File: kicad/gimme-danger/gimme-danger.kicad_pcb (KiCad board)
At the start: 4 copper layers, 46.1 x 30 mm, 74 parts, among them J3 Screw_Terminal_01x06, Q1 AO3400A, Q2 AO3400A, Q3 AO3400A, Q4 AO3400A, U1 ESP32-S3-WROOM-1, U2 TPD6S300RUKR, U3 U261-241N-4BS2SS, U4 AO4407A, U5 SKRKAEE020, U6 DDTC143EUA, U7 SKRKAEE020, U8 TPS54302

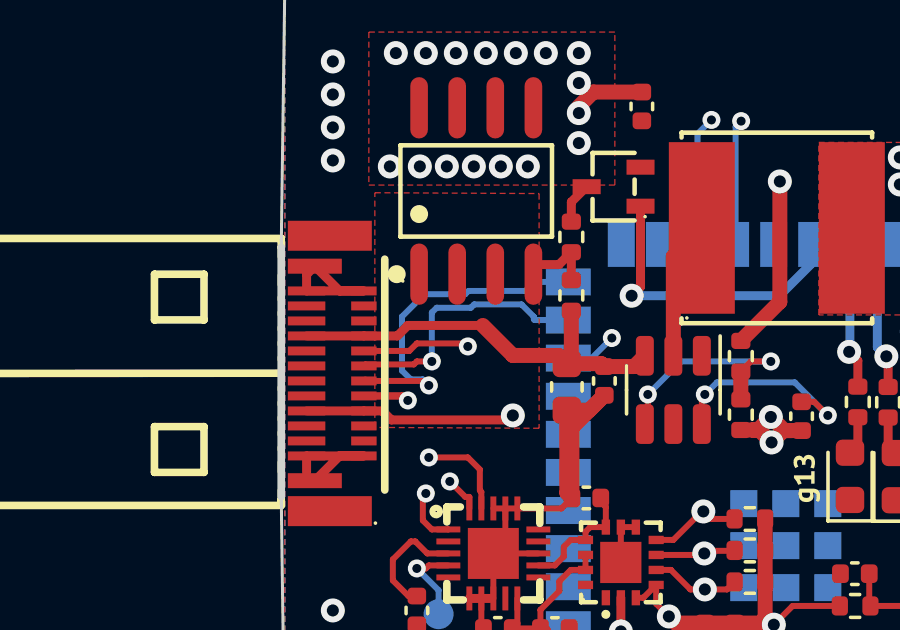
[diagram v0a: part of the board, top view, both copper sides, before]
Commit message: Moar VBus zone
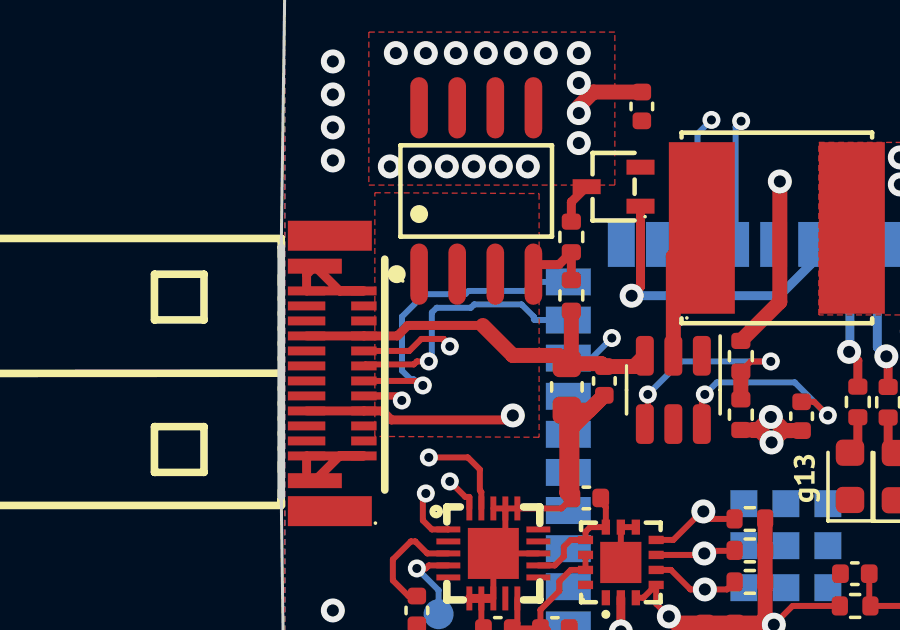
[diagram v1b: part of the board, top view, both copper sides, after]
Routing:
- net D+: track 17.3 -> 16.7 mm
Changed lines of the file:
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@@
   (segment (start 87.95 108.95) (end 87.59 109.31) (width 0.2) (layer "B.Cu") (net 61))
   (segment (start 67.5 115.9) (end 67.550406 115.950406) (width 0.2) (layer "F.Cu") (net 62))
-  (segment (start 65.8 112.4) (end 65.650064 112.250064) (width 0.2) (layer "F.Cu") (net 62))
+  (segment (start 65.350064 112.250064) (end 65.5 112.4) (width 0.2) (layer "F.Cu") (net 62))
   (segment (start 65.8 114.8) (end 67.1 114.8) (width 0.2) (layer "F.Cu") (net 62))
-  (segment (start 63.635001 112.250064) (end 63.685065 112.2) (width 0.2) (layer "F.Cu") (net 62))
+  (segment (start 63.635001 112.250064) (end 65.350064 112.250064) (width 0.2) (layer "F.Cu") (net 62))
   (segment (start 67.5 115.2) (end 67.5 115.9) (width 0.2) (layer "F.Cu") (net 62))
   (segment (start 67.550406 115.950406) (end 67.550406 116.5) (width 0.2) (layer "F.Cu") (net 62))
   (segment (start 67.1 114.8) (end 67.5 115.2) (width 0.2) (layer "F.Cu") (net 62))
-  (segment (start 65.8 112.2) (end 66 112.4) (width 0.2) (layer "F.Cu") (net 62))
-  (segment (start 65.650064 112.250064) (end 63.635001 112.250064) (width 0.2) (layer "F.Cu") (net 62))
   (via (at 65.8 114.8) (size 0.6) (drill 0.3) (layers "F.Cu" "B.Cu") (net 62))
-  (via (at 65.8 112.4) (size 0.6) (drill 0.3) (layers "F.Cu" "B.Cu") (net 62))
+  (via (at 65.6 112.4) (size 0.6) (drill 0.3) (layers "F.Cu" "B.Cu") (net 62))
+  (segment (start 65.8 112.4) (end 65.5 112.4) (width 0.2) (layer "In2.Cu") (net 62))
   (segment (start 66.1 112.7) (end 66.1 114.5) (width 0.2) (layer "In2.Cu") (net 62))
+  (segment (start 66.1 112.7) (end 65.8 112.4) (width 0.2) (layer "In2.Cu") (net 62))
   (segment (start 66.1 114.5) (end 65.8 114.8) (width 0.2) (layer "In2.Cu") (net 62))
-  (segment (start 66.1 112.7) (end 65.8 112.4) (width 0.2) (layer "In2.Cu") (net 62))
   (segment (start 65.2 112.2) (end 64.905 111.905) (width 0.2) (layer "B.Cu") (net 62))
-  (segment (start 65.8 112.4) (end 65.6 112.2) (width 0.2) (layer "B.Cu") (net 62))
   (segment (start 69.02498 109.250019) (end 69.324999 108.95) (width 0.2) (layer "B.Cu") (net 62))
   (segment (start 65.65 109.36) (end 67.01368 109.36) (width 0.2) (layer "B.Cu") (net 62))
-  (segment (start 65.6 112.2) (end 65.2 112.2) (width 0.2) (layer "B.Cu") (net 62))
+  (segment (start 65.3 112.2) (end 65.5 112.4) (width 0.2) (layer "B.Cu") (net 62))
   (segment (start 67.123661 109.250019) (end 69.02498 109.250019) (width 0.2) (layer "B.Cu") (net 62))
   (segment (start 67.01368 109.36) (end 67.123661 109.250019) (width 0.2) (layer "B.Cu") (net 62))
@@
   (segment (start 64.905 111.905) (end 64.905 110.105) (width 0.2) (layer "B.Cu") (net 62))
   (segment (start 64.905 110.105) (end 65.65 109.36) (width 0.2) (layer "B.Cu") (net 62))
+  (segment (start 65.2 112.2) (end 65.3 112.2) (width 0.2) (layer "B.Cu") (net 62))
   (segment (start 67.150355 116.116041) (end 67.150355 116.5) (width 0.2) (layer "F.Cu") (net 63))
   (segment (start 67.016041 116.116041) (end 66.5 115.6) (width 0.2) (layer "F.Cu") (net 63))
@@
   (segment (start 67.150355 116.116041) (end 67.016041 116.116041) (width 0.2) (layer "F.Cu") (net 63))
   (via (at 66.5 115.6) (size 0.6) (drill 0.3) (layers "F.Cu" "B.Cu") (net 63))
-  (via (at 65.9 111.6) (size 0.6) (drill 0.3) (layers "F.Cu" "B.Cu") (net 63))
-  (segment (start 66.5 111.8) (end 66.5 115.6) (width 0.2) (layer "In2.Cu") (net 63))
-  (segment (start 66.3 111.6) (end 66.5 111.8) (width 0.2) (layer "In2.Cu") (net 63))
-  (segment (start 65.9 111.6) (end 66.3 111.6) (width 0.2) (layer "In2.Cu") (net 63))
+  (via (at 65.8 111.6) (size 0.6) (drill 0.3) (layers "F.Cu" "B.Cu") (net 63))
+  (segment (start 66.5 115.6) (end 66.5 112.3) (width 0.2) (layer "In2.Cu") (net 63))
+  (segment (start 66.5 112.3) (end 65.8 111.6) (width 0.2) (layer "In2.Cu") (net 63))
   (segment (start 67.20005 109.81) (end 66.06 109.81) (width 0.2) (layer "B.Cu") (net 63))
   (segment (start 69.3 110.195001) (end 69.3 110.11005) (width 0.2) (layer "B.Cu") (net 63))
@@
   (segment (start 67.31005 109.7) (end 67.20005 109.81) (width 0.2) (layer "B.Cu") (net 63))
   (segment (start 69.324999 110.22) (end 69.3 110.195001) (width 0.2) (layer "B.Cu") (net 63))
-  (segment (start 64.949936 112.749936) (end 65.1 112.9) (width 0.25) (layer "F.Cu") (net 64))
   (segment (start 65.7 118.5) (end 65.4 118.5) (width 0.2) (layer "F.Cu") (net 64))
   (segment (start 63.635001 112.749936) (end 64.949936 112.749936) (width 0.25) (layer "F.Cu") (net 64))
   (segment (start 66.45033 118.400178) (end 65.799822 118.400178) (width 0.2) (layer "F.Cu") (net 64))
   (segment (start 65.799822 118.400178) (end 65.7 118.5) (width 0.2) (layer "F.Cu") (net 64))
-  (via (at 65.1 112.9) (size 0.6) (drill 0.3) (layers "F.Cu" "B.Cu") (net 64))
+  (via (at 64.9 112.9) (size 0.6) (drill 0.3) (layers "F.Cu" "B.Cu") (net 64))
   (via (at 65.4 118.5) (size 0.6) (drill 0.3) (layers "F.Cu" "B.Cu") (net 64))
+  (segment (start 65.1 113.1) (end 64.9 112.9) (width 0.2) (layer "In2.Cu") (net 64))
+  (segment (start 65.1 118.1) (end 65.1 113.1) (width 0.2) (layer "In2.Cu") (net 64))
   (segment (start 65.1 118.1) (end 65.4 118.4) (width 0.2) (layer "In2.Cu") (net 64))
-  (segment (start 65.1 112.9) (end 65.1 118.1) (width 0.2) (layer "In2.Cu") (net 64))
   (segment (start 66.125 120.025) (end 66.125 119.225) (width 0.2) (layer "B.Cu") (net 64))
   (segment (start 66.125 119.225) (end 65.4 118.5) (width 0.2) (layer "B.Cu") (net 64))
   (segment (start 66.450305 117.2) (end 65.9 117.2) (width 0.2) (layer "F.Cu") (net 66))
-  (segment (start 65.4 111) (end 67 111) (width 0.2) (layer "F.Cu") (net 66))
+  (segment (start 66.3 110.9) (end 66.5 111.1) (width 0.2) (layer "F.Cu") (net 66))
+  (segment (start 65.55 110.85) (end 66.3 110.85) (width 0.2) (layer "F.Cu") (net 66))
   (segment (start 65.9 117.2) (end 65.6 116.9) (width 0.2) (layer "F.Cu") (net 66))
   (segment (start 65.6 116.1) (end 65.7 116) (width 0.2) (layer "F.Cu") (net 66))
+  (segment (start 65.149936 111.250064) (end 65.55 110.85) (width 0.2) (layer "F.Cu") (net 66))
+  (segment (start 63.635001 111.250064) (end 65.149936 111.250064) (width 0.2) (layer "F.Cu") (net 66))
   (segment (start 65.6 116.9) (end 65.6 116.1) (width 0.2) (layer "F.Cu") (net 66))
   (segment (start 66.45033 117.200025) (end 66.450305 117.2) (width 0.2) (layer "F.Cu") (net 66))
-  (segment (start 67 111) (end 67.1 111.1) (width 0.2) (layer "F.Cu") (net 66))
-  (segment (start 65.149936 111.250064) (end 65.4 111) (width 0.2) (layer "F.Cu") (net 66))
-  (segment (start 63.635001 111.250064) (end 65.149936 111.250064) (width 0.2) (layer "F.Cu") (net 66))
+  (segment (start 66.3 110.85) (end 66.3 110.9) (width 0.2) (layer "F.Cu") (net 66))
   (via (at 65.7 116) (size 0.6) (drill 0.3) (layers "F.Cu" "B.Cu") (net 66))
-  (via (at 67.1 111.1) (size 0.6) (drill 0.3) (layers "F.Cu" "B.Cu") (net 66))
+  (via (at 66.5 111.1) (size 0.6) (drill 0.3) (layers "F.Cu" "B.Cu") (net 66))
+  (segment (start 66.9 114.7) (end 66.9 111.2) (width 0.2) (layer "In2.Cu") (net 66))
+  (segment (start 66.6 111.2) (end 66.5 111.1) (width 0.2) (layer "In2.Cu") (net 66))
   (segment (start 66.7 116.5) (end 66.2 116.5) (width 0.2) (layer "In2.Cu") (net 66))
-  (segment (start 67.1 111.1) (end 66.9 111.3) (width 0.2) (layer "In2.Cu") (net 66))
   (segment (start 66.2 116.5) (end 65.7 116) (width 0.2) (layer "In2.Cu") (net 66))
   (segment (start 67.1 114.9) (end 67.1 116.1) (width 0.2) (layer "In2.Cu") (net 66))
-  (segment (start 66.9 111.3) (end 66.9 114.7) (width 0.2) (layer "In2.Cu") (net 66))
   (segment (start 67.1 116.1) (end 66.7 116.5) (width 0.2) (layer "In2.Cu") (net 66))
   (segment (start 66.9 114.7) (end 67.1 114.9) (width 0.2) (layer "In2.Cu") (net 66))
+  (segment (start 66.9 111.2) (end 66.6 111.2) (width 0.2) (layer "In2.Cu") (net 66))
   (segment (start 74.9 113.6875) (end 74.9 112.8) (width 0.2) (layer "F.Cu") (net 67))
   (segment (start 78.645 112.945) (end 79.1 113.4) (width 0.2) (layer "F.Cu") (net 67))
@@
         (xy 64 105.976632)
         (xy 69.475742 106.004229)
-        (xy 69.475742 113.827597)
-        (xy 64 113.8)
-      )
-    )
+        (xy 69.475742 114.127597)
+        (xy 64 114.1)
+      )
+    )
